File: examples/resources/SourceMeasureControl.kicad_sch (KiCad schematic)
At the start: 19 parts

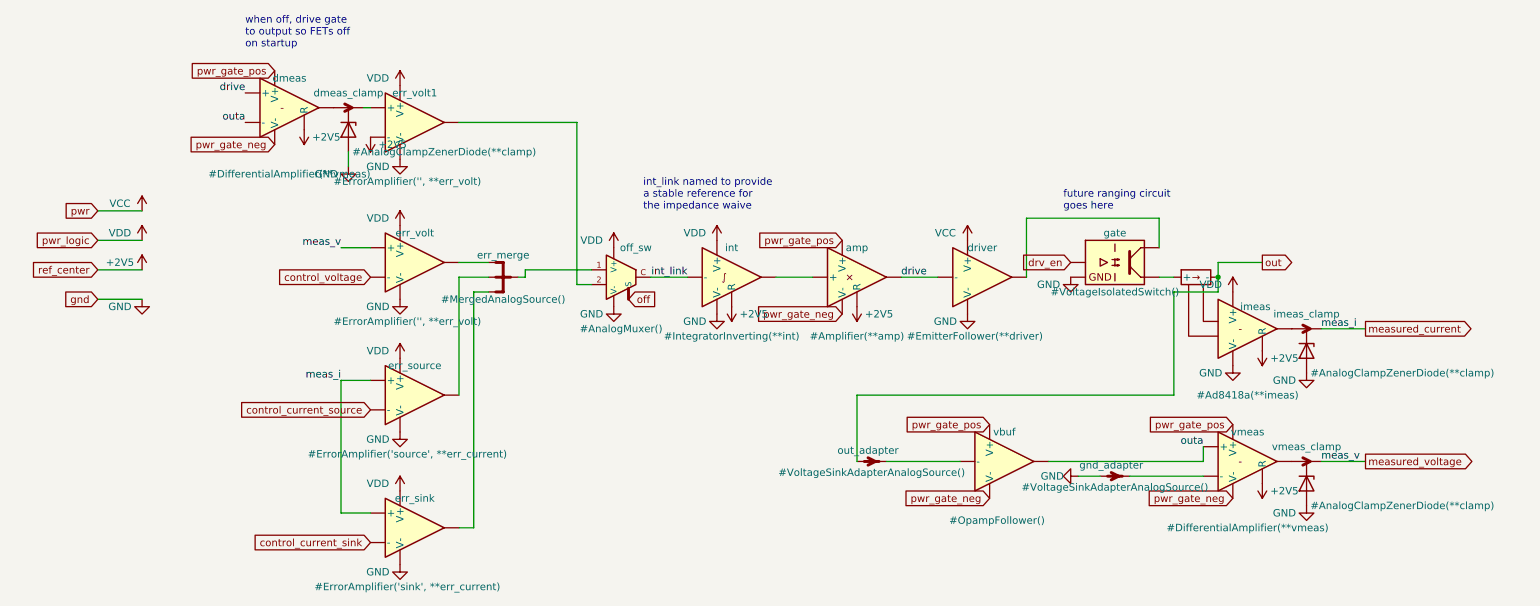
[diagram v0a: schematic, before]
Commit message: wip clamp dev
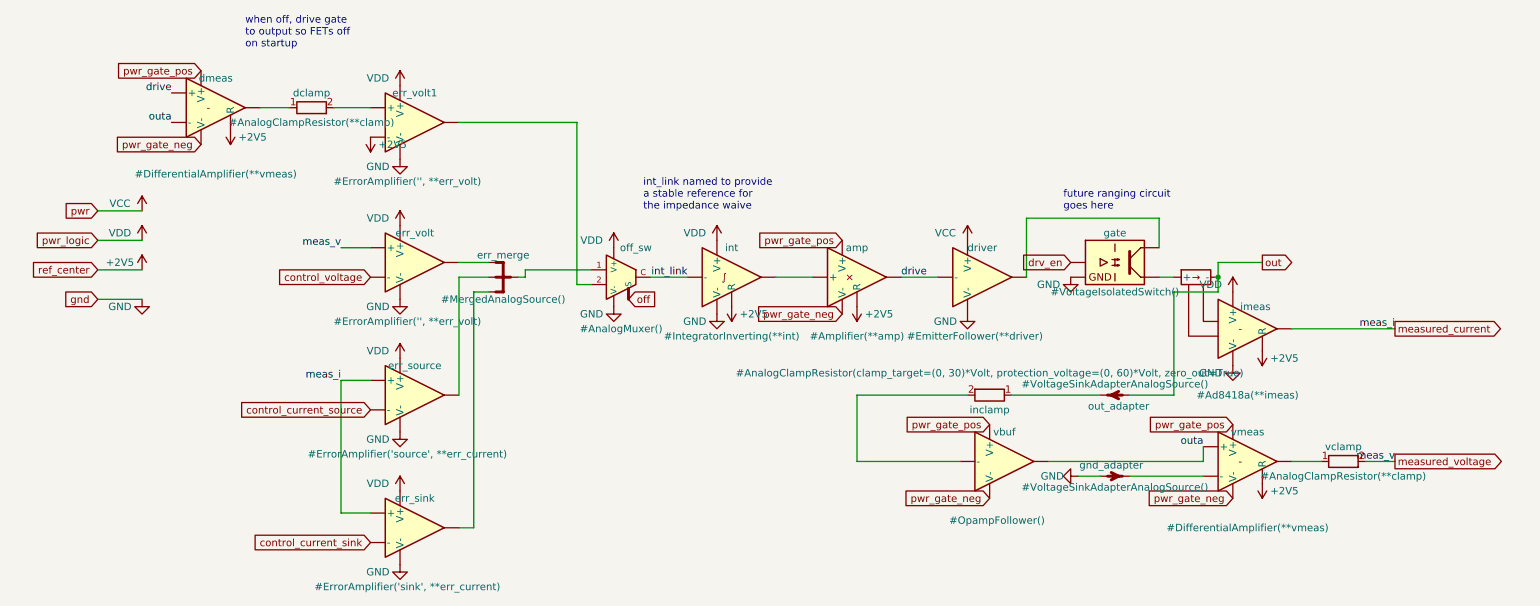
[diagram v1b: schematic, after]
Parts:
- removed dmeas_clamp, imeas_clamp, vmeas_clamp: #AnalogClampZenerDiode(**clamp), symbol edg_importable:AnalogClampZenerDiode
- added dclamp, vclamp: #AnalogClampResistor(**clamp), symbol Device:R
- added inclamp: #AnalogClampResistor(clamp_target=(0, 30)*Volt, p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, symbol Device:R
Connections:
- net measured_current: now also imeas.3
- net measured_voltage: now also vclamp.2
- net at dmeas.3: now also dclamp.1
- net at vmeas.3: now also vclamp.1
- net at out_adapter.2: now also inclamp.1; no longer vbuf.1 (-)
- net at err_volt1.1 (+): now also dclamp.2
- new net: inclamp.2, vbuf.1 (-)
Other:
- moved on the sheet: dmeas, out_adapter
